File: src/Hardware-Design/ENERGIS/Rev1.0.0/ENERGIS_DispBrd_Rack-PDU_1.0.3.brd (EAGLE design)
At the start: 124 x 28 mm, 80 parts, among them CON1 DNI, CON2 AFC11-S20ICC-00, IC1 MCP23017T-E/ML, IC2 MCP23017T-E/ML, T1 BSS138

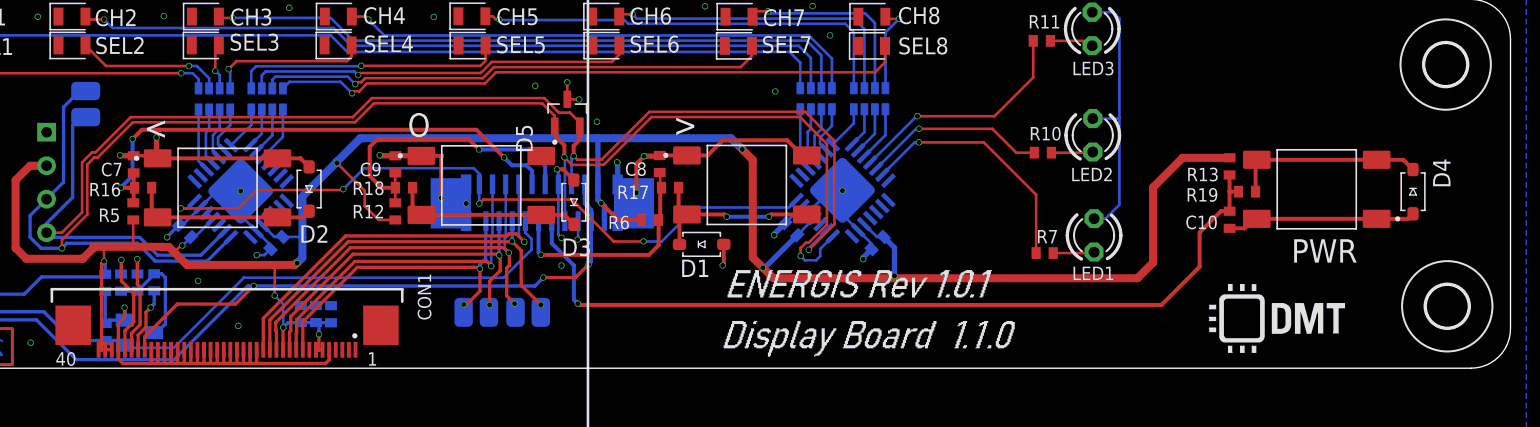
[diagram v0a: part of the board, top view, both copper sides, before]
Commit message: update documentation
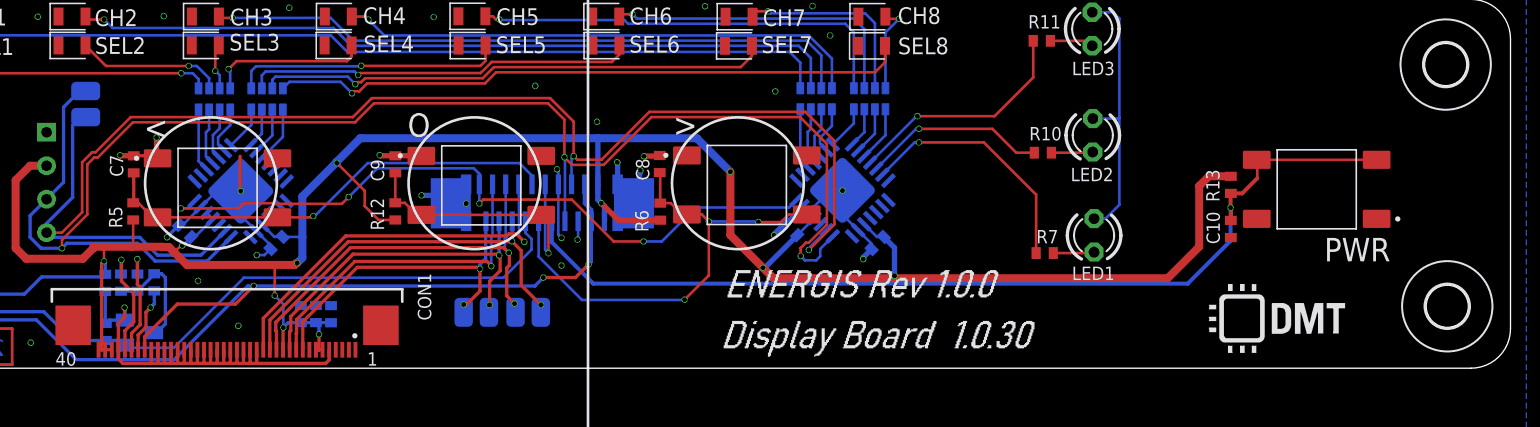
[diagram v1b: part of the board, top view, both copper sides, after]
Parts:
- removed D1, D2, D3, D4: PTVS3V3S1UR,115, ds_diode:SOD-123
- removed D5: RCLAMP0582BQTCT, ds_diode:SOT-523
- removed R16, R17, R18, R19: 10K 1%, ds_resistor:0402
- R12, R13, R5, R6: value 33K 1% -> 10K 1%
- moved R13 1.40 mm to (106.8, 37.9)
- moved R6 1.00 mm to (63.5, 35.9), turned to 90 degrees
- moved C10 0.71 mm to (106.8, 34.6)
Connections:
- removed net N$24: D3.C, O.3, O.4, R18.1
- removed net N$25: D4.C, PWR.3, PWR.4, R19.1
- removed net N$26: >.3, >.4, D1.C, R17.1
- removed net N$7: <.3, <.4, D2.C, R16.1
- net GND: no longer D1.A, D2.A, D3.A, D4.A, D5.3
- net I2C0_SCL: no longer D5.1
- net I2C0_SDA: no longer D5.2
- net KEY_0: now also <.3, <.4; no longer R16.2
- net KEY_1: now also >.3, >.4; no longer R17.2
- net KEY_2: now also O.3, O.4; no longer R18.2
- net KEY_3: now also PWR.3, PWR.4; no longer R19.2
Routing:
- net GND: track 169.3 -> 123.6 mm, vias 40 -> 37
- net KEY_1: track 17.6 -> 36.2 mm, vias 1 -> 3
- net N$25: track 14.6 -> 0.00 mm
- net N$24: track 14.2 -> 0.00 mm
- net N$7: track 14.1 -> 0.00 mm
- net N$26: track 14.1 -> 0.00 mm, vias 2 -> 0
- net KEY_3: track 64.5 -> 73.4 mm
- net KEY_0: track 40.7 -> 35.8 mm, vias 3 -> 1
- net +3V3: track 200.4 -> 199.2 mm
- net I2C0_SDA: track 111.3 -> 110.7 mm
- net KEY_2: track 22.8 -> 22.2 mm
